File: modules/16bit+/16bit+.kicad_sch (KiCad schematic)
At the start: 52 parts, among them J1 Conn_01x08_Socket, J2 Conn_01x08_Socket, J5 USB_C_Receptacle_USB2.0_14P, SW1 K2-1808SN-A4SW-01, SW2 K2-1808SN-A4SW-01, SW3 K2-1808SN-A4SW-01, U1 RP2350_60QFN, U2 W25Q128JVS, U3 MCP6002-xSN, U5 PSRAM, Y1 ABM8-272-T3

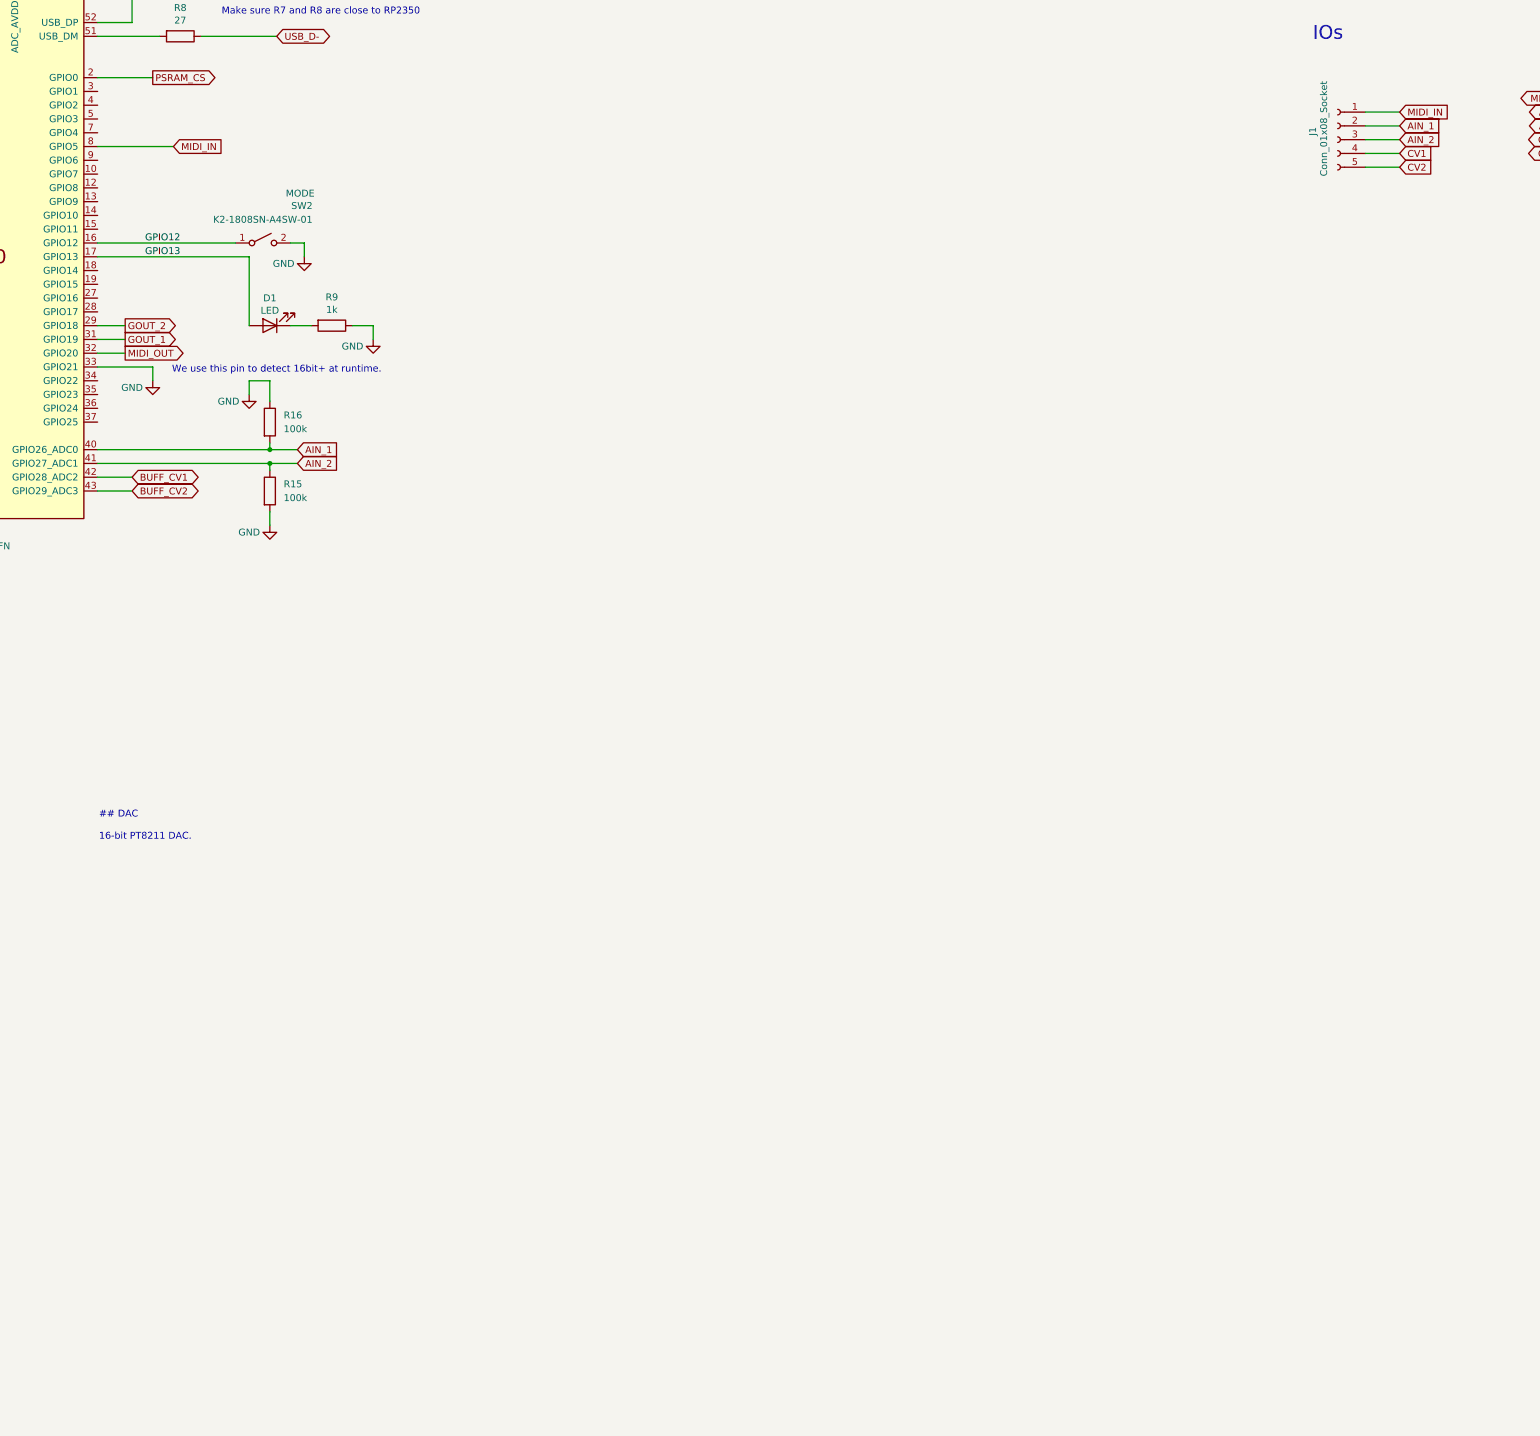
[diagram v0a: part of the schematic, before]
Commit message: Finalize the schematics
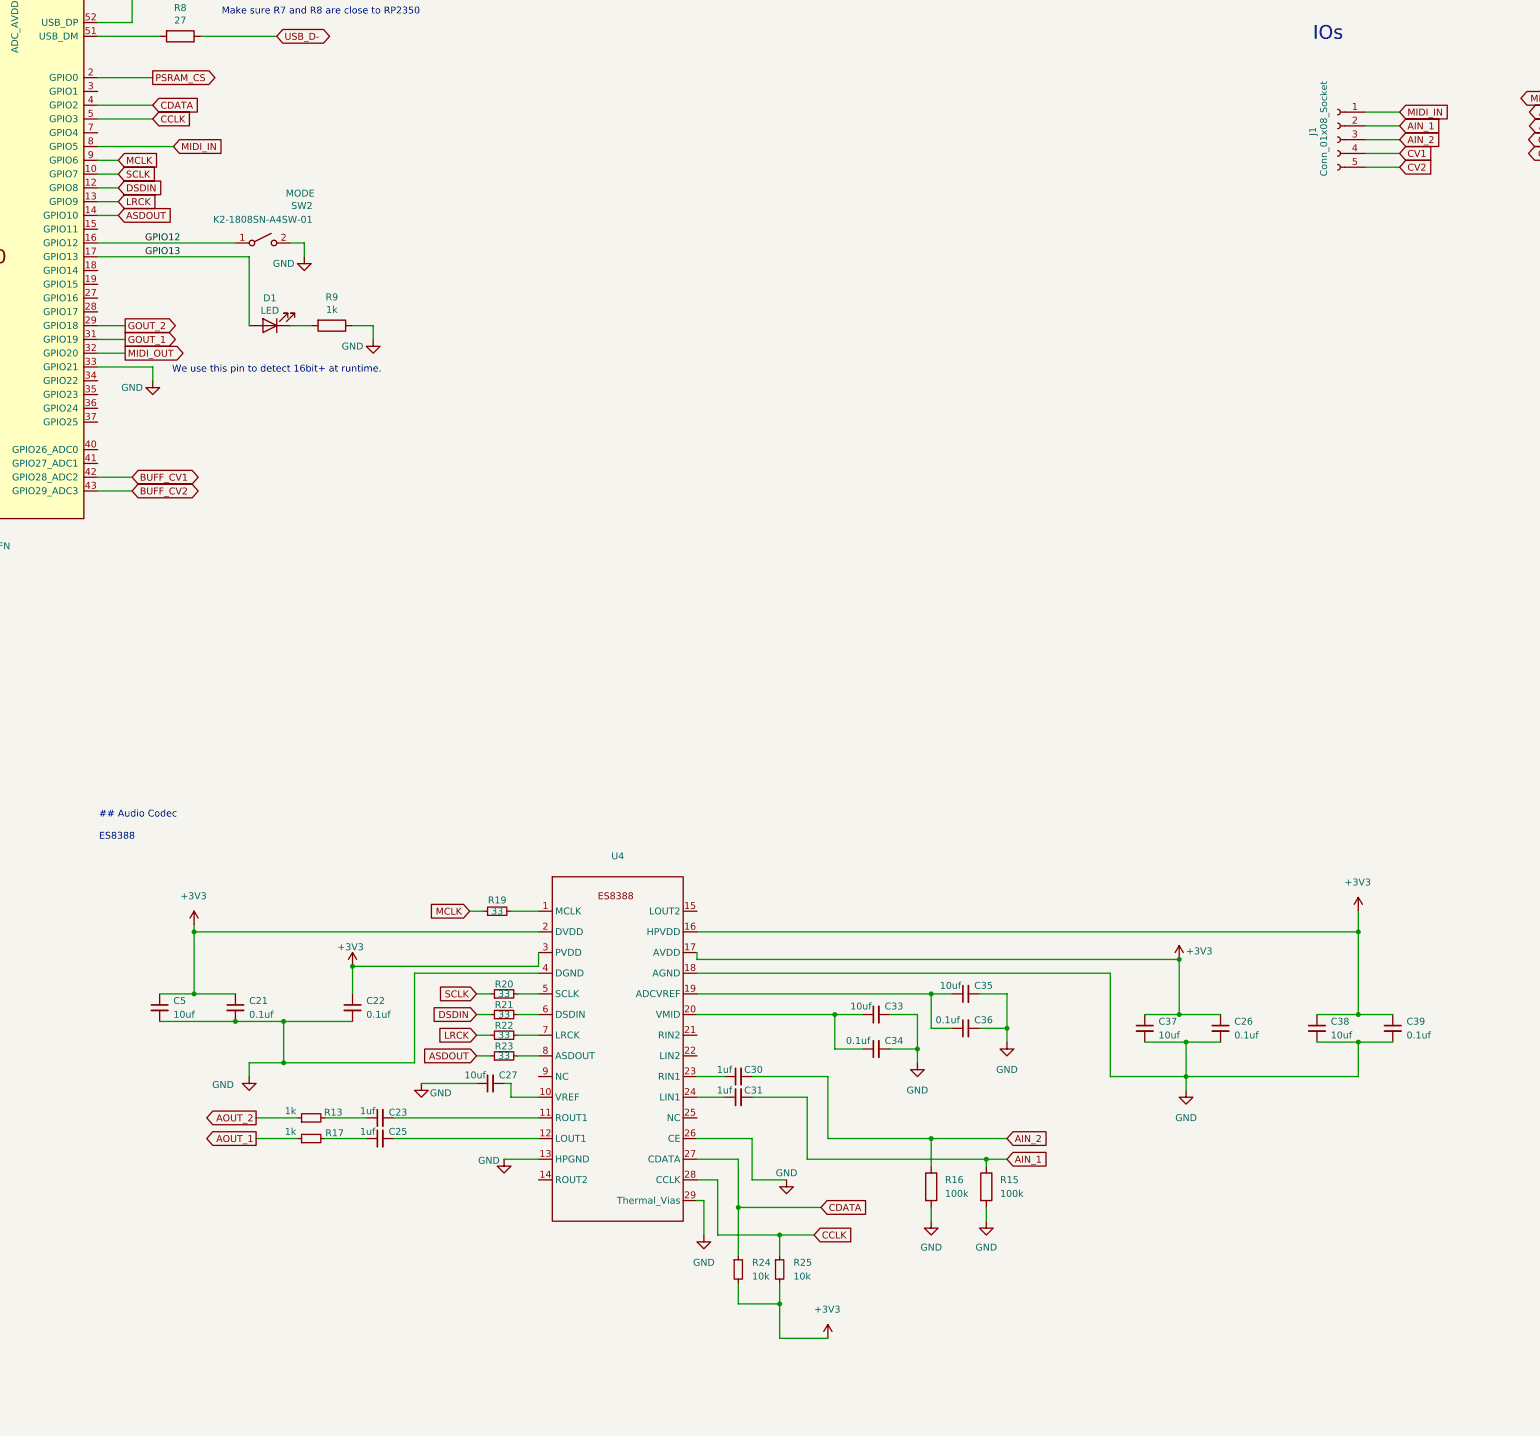
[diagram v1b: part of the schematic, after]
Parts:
- added C21, C22, C26, C34, C36, C39: 0.1uf, Capacitor_SMD:C_0402_1005Metric, symbol Device:C_Small
- added C23, C25, C30, C31: 1uf, Capacitor_SMD:C_0402_1005Metric, symbol Device:C_Small
- added C27, C33, C35, C37, C38, C5: 10uf, Capacitor_SMD:C_0402_1005Metric, symbol Device:C_Small
- added R13, R17: 1k, Resistor_SMD:R_0402_1005Metric, symbol Device:R_Small
- added R19, R20, R21, R22, R23: 33, Resistor_SMD:R_0402_1005Metric, symbol Device:R_Small
- added R24, R25: 10k, Resistor_SMD:R_0402_1005Metric, symbol Device:R_Small
- added U4: ~, Package_DFN_QFN:QFN-28-1EP_4x4mm_P0.45mm_EP2.4x2.4mm_ThermalVias, symbol BreadModular_Symbols:ES8388
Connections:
- net +3V3: now also C21.1, C22.1, C26.1, C37.1, C38.1, C39.1, C5.1, R24.2, R25.2, U4.16 (HPVDD), U4.17 (AVDD), U4.2 (DVDD), U4.3 (PVDD)
- net AIN_1: now also R15.1, C31.2; no longer R16.2, U1.40 (GPIO26_ADC0)
- net AIN_2: now also R16.1, C30.2; no longer R15.1, U1.41 (GPIO27_ADC1)
- net AOUT_1: now also R17.1
- net AOUT_2: now also R13.1
- net GND: now also R16.2, C21.2, C22.2, C26.2, C27.1, C33.2, C34.2, C35.2, C36.2, C37.2, C38.2, C39.2, C5.2, U4.13 (HPGND), U4.18 (AGND), U4.26 (CE), U4.29 (Thermal_Vias), U4.4 (DGND); no longer R16.1
- net SCLK: now reaches U1.10 (GPIO7)
- net SCLK: now also R20.1
- net DSDIN: now reaches U1.12 (GPIO8)
- net DSDIN: now also R21.1
- net LRCK: now reaches U1.13 (GPIO9)
- net LRCK: now also R22.1
- net ASDOUT: now reaches U1.14 (GPIO10)
- net ASDOUT: now also R23.1
- net CDATA: now reaches U1.4 (GPIO2)
- net CDATA: now also R24.1, U4.27 (CDATA)
- net CCLK: now reaches U1.5 (GPIO3)
- net CCLK: now also R25.1, U4.28 (CCLK)
- net MCLK: now reaches U1.9 (GPIO6)
- net MCLK: now also R19.1
- new net: C23.1, R13.2
- new net: C30.1, U4.23 (RIN1)
- new net: C23.2, U4.11 (ROUT1)
- new net: R20.2, U4.5 (SCLK)
- new net: R22.2, U4.7 (LRCK)
- new net: R19.2, U4.1 (MCLK)
- new net: C33.1, C34.1, U4.20 (VMID)
- new net: C25.1, R17.2
- new net: C27.2, U4.10 (VREF)
- new net: C31.1, U4.24 (LIN1)
- new net: R23.2, U4.8 (ASDOUT)
- new net: C35.1, C36.1, U4.19 (ADCVREF)
- new net: C25.2, U4.12 (LOUT1)
- new net: R21.2, U4.6 (DSDIN)
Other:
- note added: "## Audio Codec ES8388"
- note removed: "## DAC 16-bit PT8211 DAC."
- moved on the sheet: R15, R16
